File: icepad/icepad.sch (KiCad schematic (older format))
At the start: 41 parts, among them SW1 SW_DIP_x01, SW10 SW_DIP_x01, SW11 SW_DIP_x01, SW12 SW_DIP_x01, SW13 SW_DIP_x01, SW14 SW_DIP_x01, SW15 SW_DIP_x01, SW16 SW_DIP_x01, SW17 SW_DIP_x01, SW18 SW_DIP_x01, SW19 SW_DIP_x01, SW2 SW_DIP_x01, SW20 SW_DIP_x01, SW3 SW_DIP_x01, SW4 SW_DIP_x01, SW5 SW_DIP_x01, SW6 SW_DIP_x01, SW7 SW_DIP_x01, SW8 SW_DIP_x01, SW9 SW_DIP_x01, U1 STM32F042F6Px

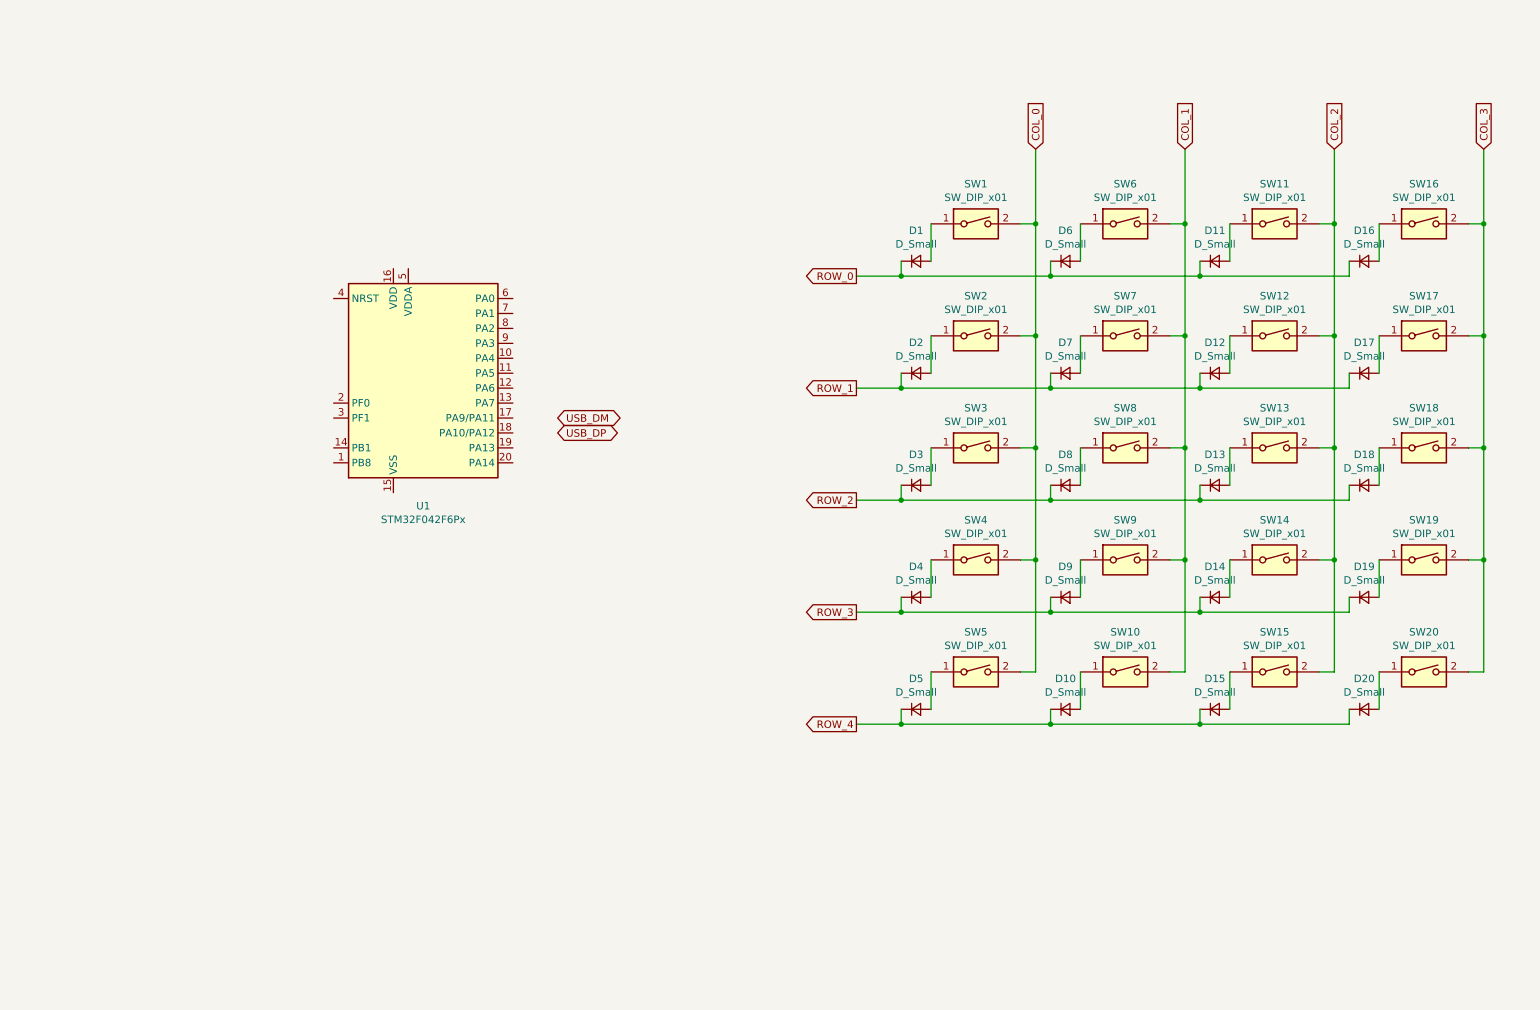
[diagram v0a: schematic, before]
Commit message: schematic edits
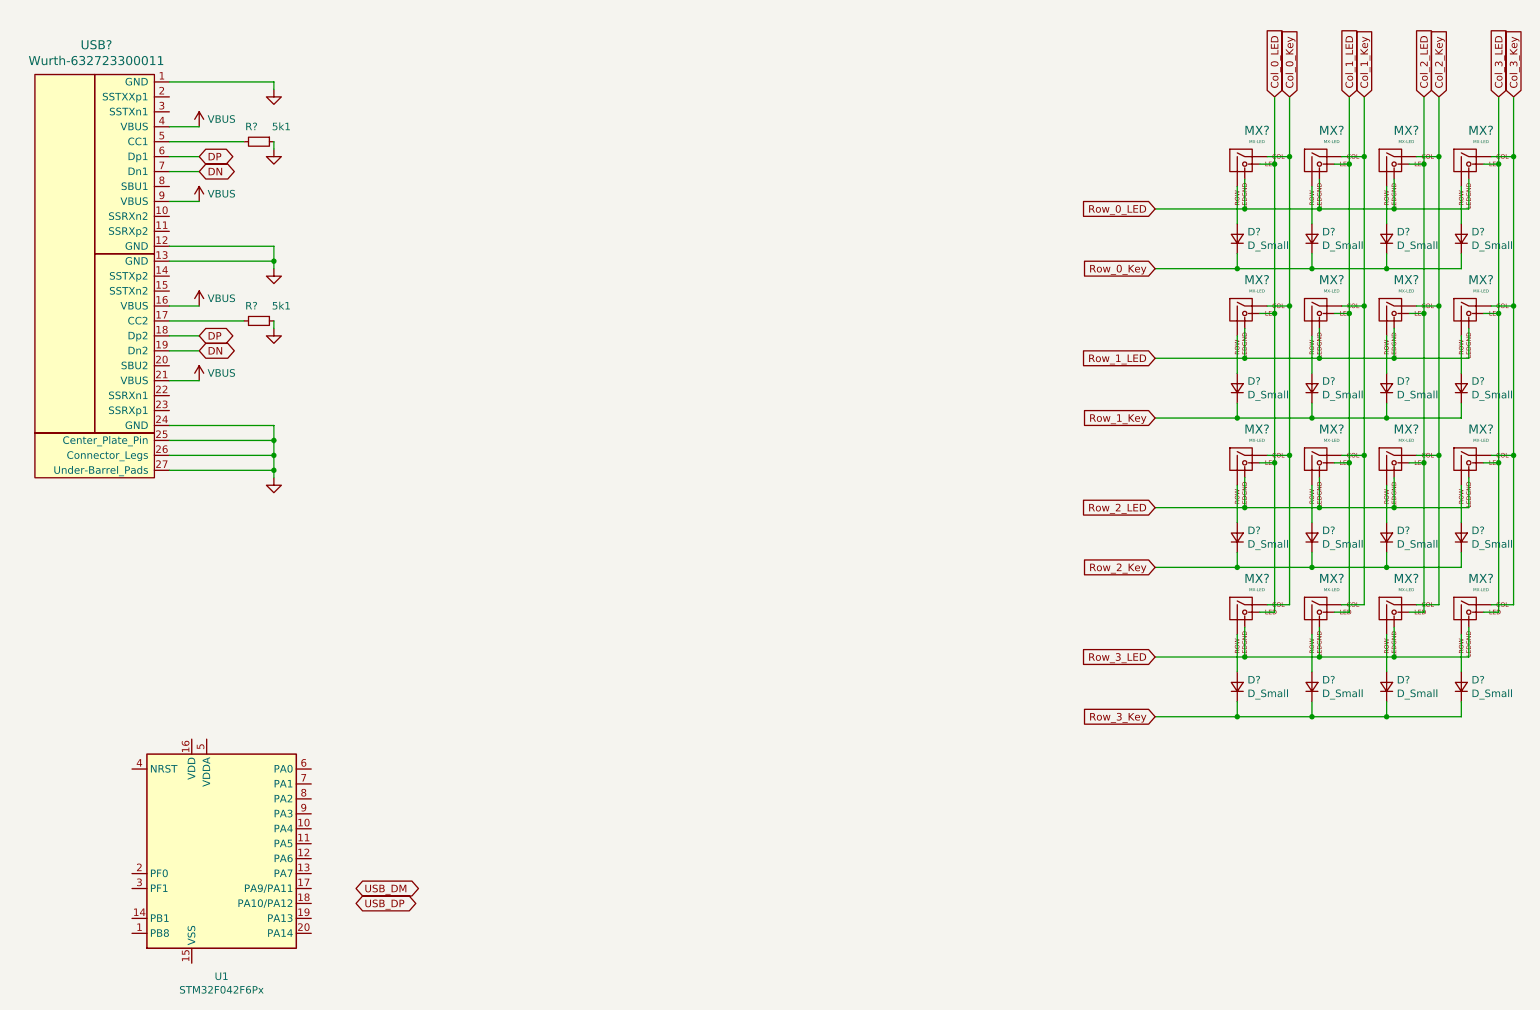
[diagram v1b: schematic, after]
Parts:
- removed D1, D10, D11, D12, D13, D14, D15, D16, D17, D18, D19, D2, D20, D3, D4, D5, D6, D7, D8, D9: D_Small, symbol Device:D_Small
- removed SW1, SW10, SW11, SW12, SW13, SW14, SW15, SW16, SW17, SW18, SW19, SW2, SW20, SW3, SW4, SW5, SW6, SW7, SW8, SW9: SW_DIP_x01, keyswitches:Kailh_socket_MX, symbol Switch:SW_DIP_x01
- added D? (x16): D_Small, symbol Device:D_Small
- added MX? (x16): MX-LED, symbol MX_Alps_Hybrid:MX-LED
- added R? (x2): 5k1, symbol Device:R_Small
- added USB?: Wurth-632723300011, symbol Type-C:Wurth-632723300011
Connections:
- new net: D?.2 (A), MX?.2 (ROW) (x16)
- new net: R?.2, USB?.17 (CC2)
- new net: R?.2, USB?.5 (CC1)
- new net Col_0_Key: MX?.1 (COL), MX?.1 (COL), MX?.1 (COL), MX?.1 (COL)
- new net Col_0_LED: MX?.3 (LED), MX?.3 (LED), MX?.3 (LED), MX?.3 (LED)
- new net Col_1_Key: MX?.1 (COL), MX?.1 (COL), MX?.1 (COL), MX?.1 (COL)
- new net Col_1_LED: MX?.3 (LED), MX?.3 (LED), MX?.3 (LED), MX?.3 (LED)
- new net Col_2_Key: MX?.1 (COL), MX?.1 (COL), MX?.1 (COL), MX?.1 (COL)
- new net Col_2_LED: MX?.3 (LED), MX?.3 (LED), MX?.3 (LED), MX?.3 (LED)
- new net Col_3_Key: MX?.1 (COL), MX?.1 (COL), MX?.1 (COL), MX?.1 (COL)
- new net Col_3_LED: MX?.3 (LED), MX?.3 (LED), MX?.3 (LED), MX?.3 (LED)
- new net DN: USB?.19 (Dn2), USB?.7 (Dn1)
- new net DP: USB?.18 (Dp2), USB?.6 (Dp1)
- new net GND: R?.1, R?.1, USB?.1 (GND), USB?.12 (GND), USB?.13 (GND), USB?.24 (GND), USB?.25 (Center_Plate_Pin), USB?.26 (Connector_Legs), USB?.27 (Under-Barrel_Pads)
- new net Row_0_Key: D?.1 (K), D?.1 (K), D?.1 (K), D?.1 (K)
- new net Row_0_LED: MX?.4 (LEDGND), MX?.4 (LEDGND), MX?.4 (LEDGND), MX?.4 (LEDGND)
- new net Row_1_Key: D?.1 (K), D?.1 (K), D?.1 (K), D?.1 (K)
- new net Row_1_LED: MX?.4 (LEDGND), MX?.4 (LEDGND), MX?.4 (LEDGND), MX?.4 (LEDGND)
- new net Row_2_Key: D?.1 (K), D?.1 (K), D?.1 (K), D?.1 (K)
- new net Row_2_LED: MX?.4 (LEDGND), MX?.4 (LEDGND), MX?.4 (LEDGND), MX?.4 (LEDGND)
- new net Row_3_Key: D?.1 (K), D?.1 (K), D?.1 (K), D?.1 (K)
- new net Row_3_LED: MX?.4 (LEDGND), MX?.4 (LEDGND), MX?.4 (LEDGND), MX?.4 (LEDGND)
- new net VBUS: USB?.16 (VBUS), USB?.21 (VBUS), USB?.4 (VBUS), USB?.9 (VBUS)
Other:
- moved on the sheet: U1
